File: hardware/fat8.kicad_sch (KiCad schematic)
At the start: 27 parts, among them J1 Conn_ARM_JTAG_SWD_10, J2 USB_B_Micro, J3 Conn_02x10_Row_Letter_First, SW1 KMR241GLFS, U1 C8008, U2 FM1808B-SG, U4 ATF1504ASL-25AU100, U5 MCP2221AxSL

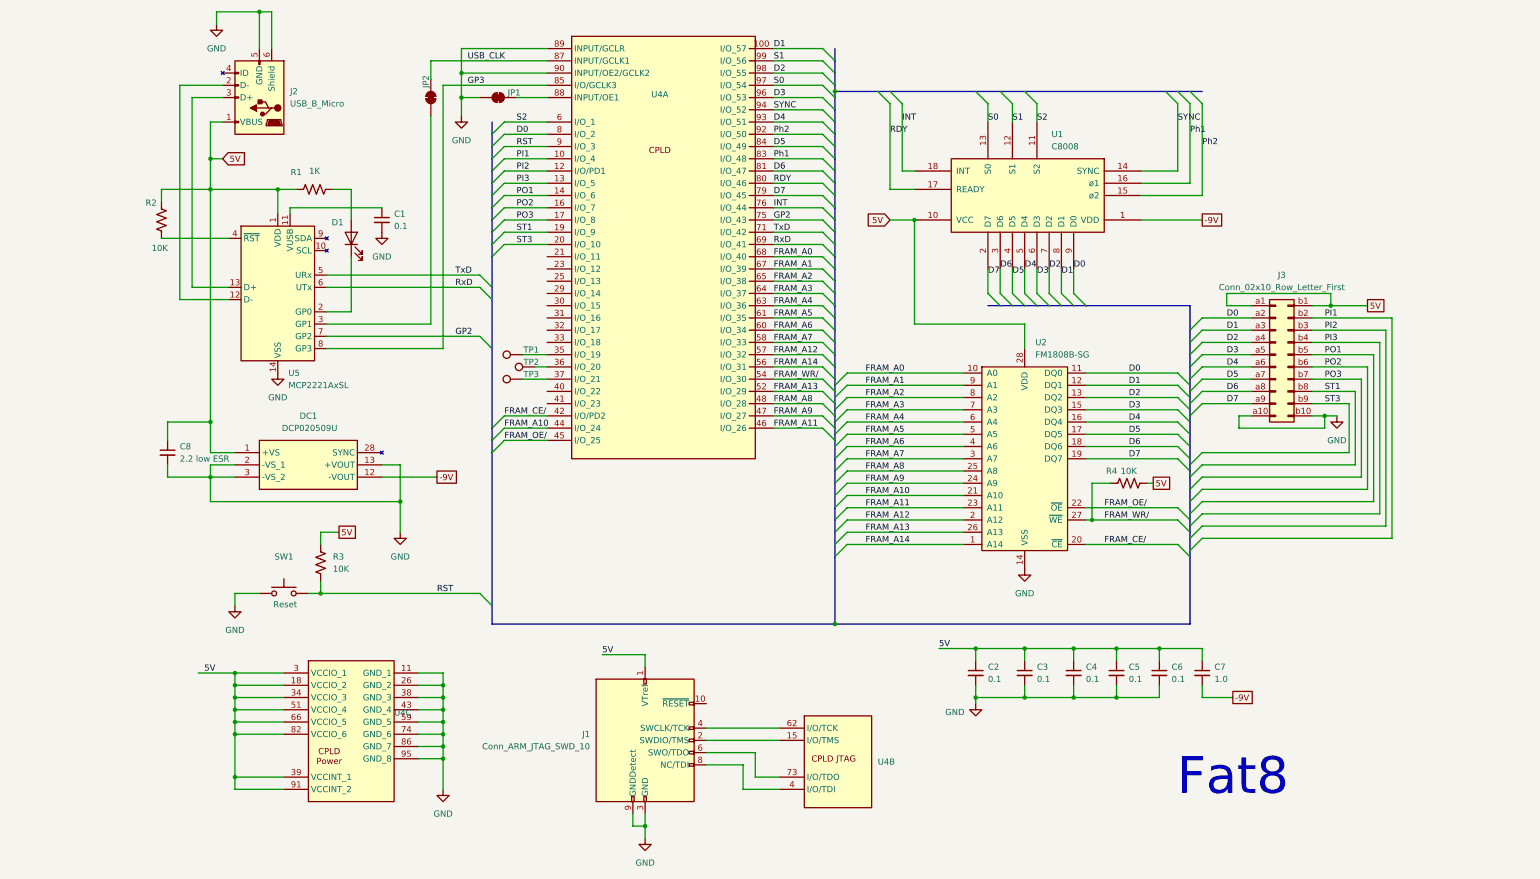
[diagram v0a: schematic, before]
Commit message: checkpoint 20250424
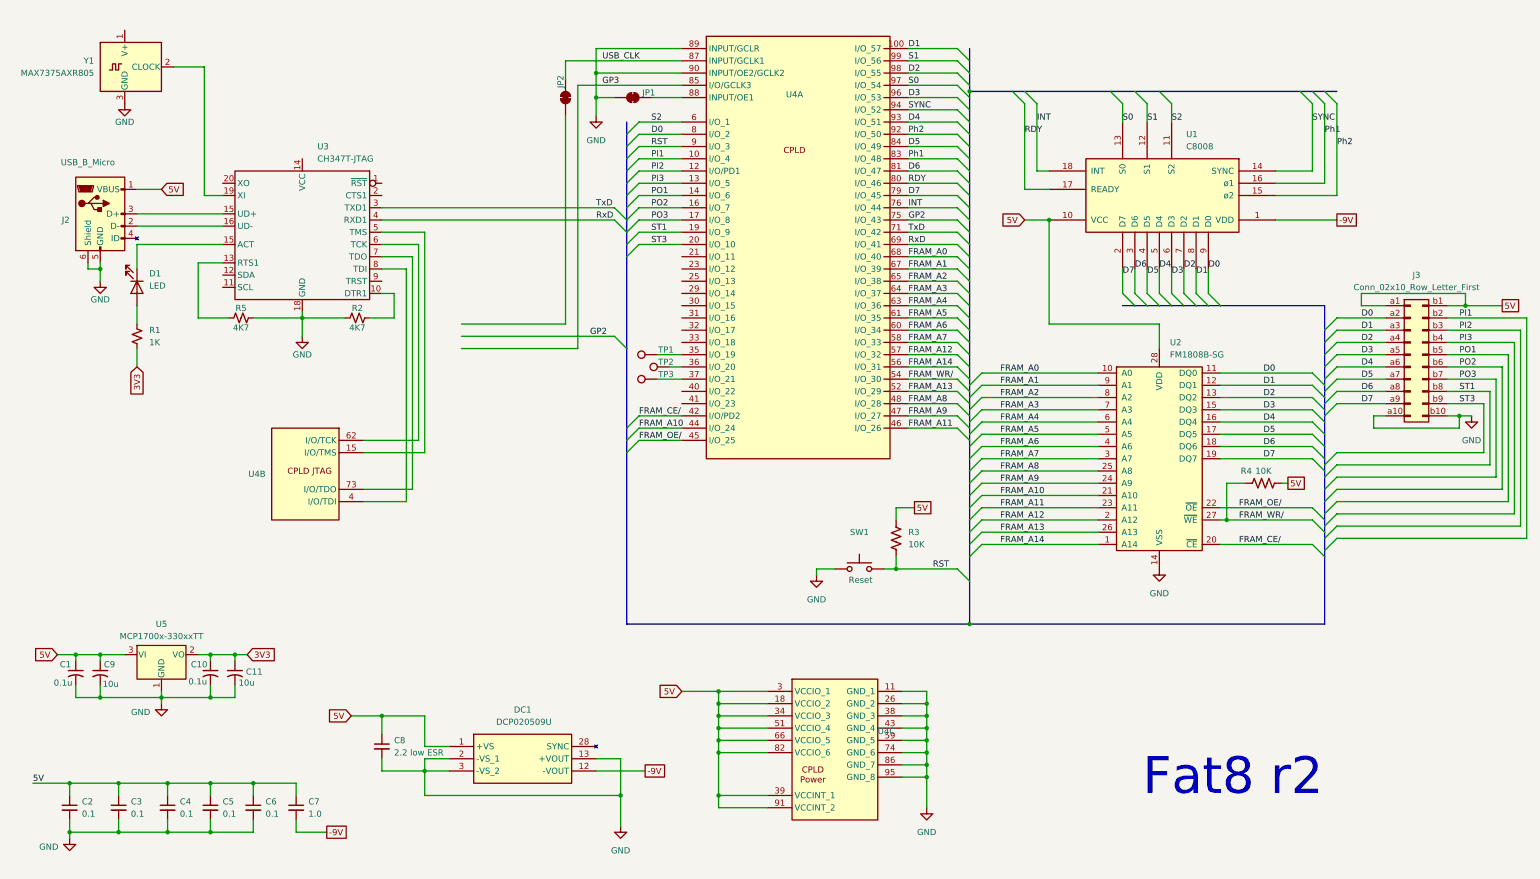
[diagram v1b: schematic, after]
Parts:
- removed C1: 0.1, Capacitor_SMD:C_0603_1608Metric, symbol Device:C_Small
- removed J1: Conn_ARM_JTAG_SWD_10, Connector_PinHeader_1.27mm:PinHeader_2x05_P1.27mm_Vertical_SMD, symbol Connector:Conn_ARM_JTAG_SWD_10
- removed R1: 1K, Resistor_SMD:R_0603_1608Metric, symbol Device:R_US
- removed R2: 10K, Resistor_SMD:R_0603_1608Metric, symbol Device:R_US
- removed U5: MCP2221AxSL, Package_SO:SOIC-14_3.9x8.7mm_P1.27mm, symbol Interface_USB:MCP2221AxSL
- added C1, C10: 0.1u, symbol Device:C_Small_US
- added C11, C9: 10u, symbol Device:C_Small_US
- added R1: 1K, symbol Device:R_Small_US
- added R2, R5: 4K7, symbol Device:R_Small_US
- added U3: CH347T-JTAG, Package_SO:TSSOP-20_4.4x6.5mm_P0.65mm, symbol fat8:CH347T-JTAG
- added U5: MCP1700x-330xxTT, Package_TO_SOT_SMD:SOT-23, symbol Regulator_Linear:MCP1700x-330xxTT
- added Y1: MAX7375AXR805, Package_TO_SOT_SMD:SOT-323_SC-70, symbol Oscillator:MAX7375AXR805
- D1: footprint Capacitor_SMD:C_0603_1608Metric -> (none)
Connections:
- net 5V: now also C1.1, C9.1, U5.3 (VI)
- net GND: now also C1.2, C10.2, C11.2, C9.2, R2.1, R5.2, U3.18 (GND), U5.1 (GND), Y1.3 (GND)
- net RxD: now also U3.4 (RXD1)
- net TxD: now also U3.3 (TXD1)
- net at J2.2 (D-): now also U3.16 (UD-)
- net at J2.3 (D+): now also U3.15 (ACT)
- net at D1.1 (K): now also U3.15 (ACT)
- net at U4.15 (I/O/TMS): now also U3.5 (TMS)
- net at U4.62 (I/O/TCK): now also U3.6 (TCK)
- net at U4.73 (I/O/TDO): now also U3.7 (TDO)
- net at U4.4 (I/O/TDI): now also U3.8 (TDI)
- net at D1.2 (A): now also R1.1
- new net: R2.2, U3.10 (DTR1)
- new net: U3.19 (XI), Y1.2 (CLOCK)
- new net: R5.1, U3.13 (RTS1)
- new net 3V3: C10.1, C11.1, R1.2, U5.2 (VO)
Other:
- note added: "Fat8 r2"
- note removed: "Fat8"
- moved on the sheet: C2, C3, C4, C5, C6, C7, C8, DC1, J2, J3, JP1, JP2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
